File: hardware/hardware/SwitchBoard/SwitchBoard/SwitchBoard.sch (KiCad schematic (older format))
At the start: 36 parts, among them SW1 SW_SPDT, SW2 SW_SPDT, SW3 SW_SPDT, SW4 SW_SPDT, SW5 SW_SPDT, SW6 SW_SPDT, SW7 SW_SPDT, SW8 SW_SPDT, U1 BeagleBone_P8, U2 MCP23S08, U3 BeagleBone_P9, U4 NCP1117-3.3_SOT223

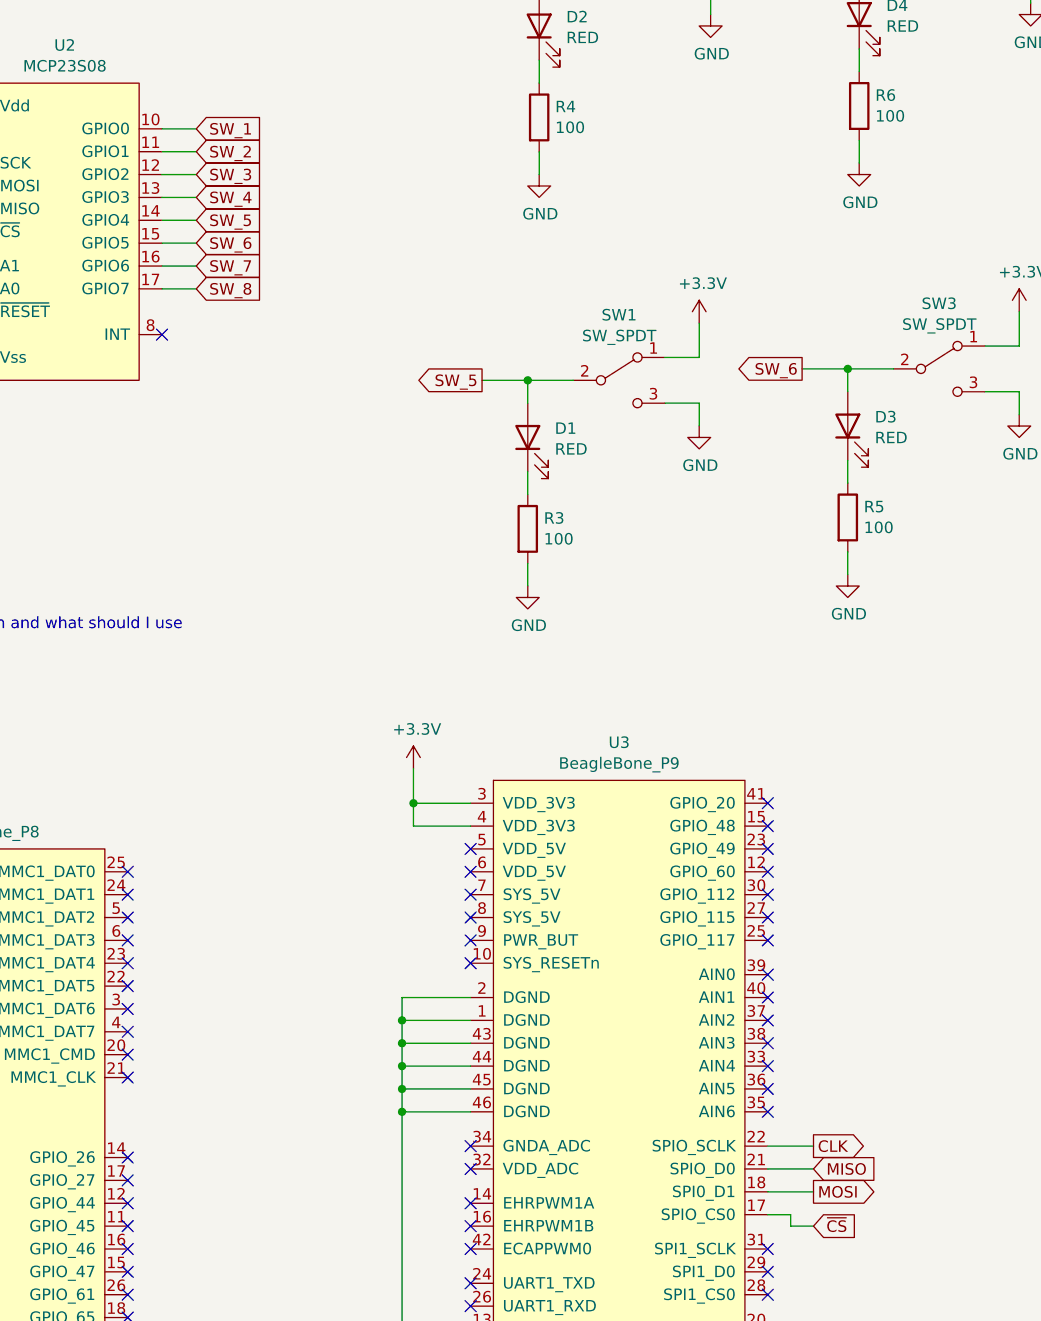
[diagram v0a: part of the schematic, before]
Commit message: More progress on switchboard
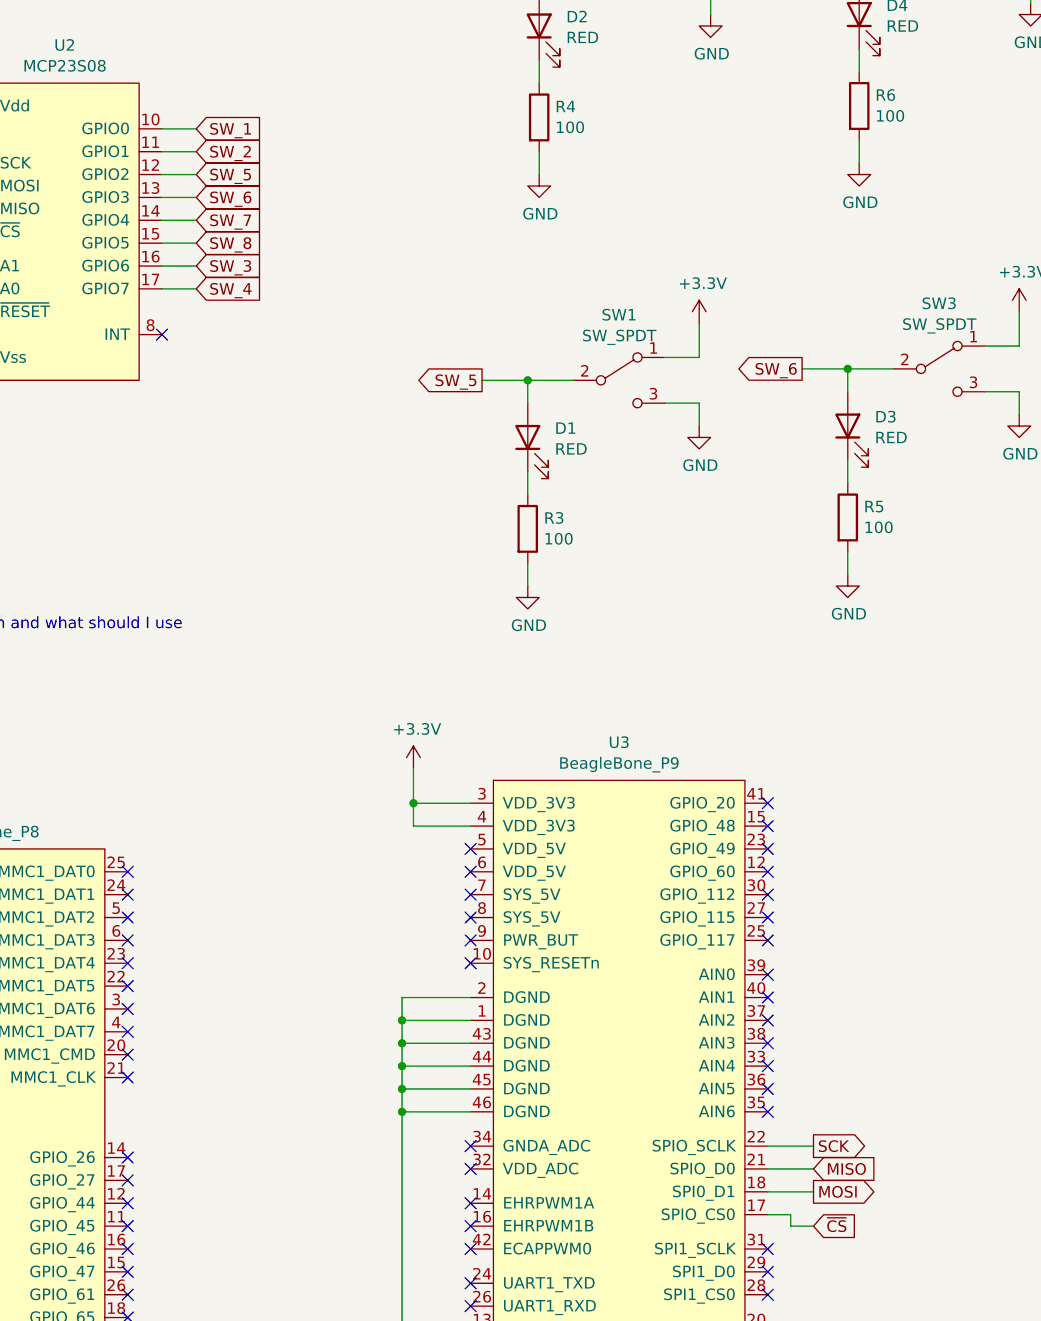
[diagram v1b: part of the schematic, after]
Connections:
- net CLK is gone; now on net SCK: U3.22 (SPIO_SCLK)
- net SW_3: now also U2.16 (GPIO6); no longer U2.12 (GPIO2)
- net SW_4: now also U2.17 (GPIO7); no longer U2.13 (GPIO3)
- net SW_5: now also U2.12 (GPIO2); no longer U2.14 (GPIO4)
- net SW_6: now also U2.13 (GPIO3); no longer U2.15 (GPIO5)
- net SW_7: now also U2.14 (GPIO4); no longer U2.16 (GPIO6)
- net SW_8: now also U2.15 (GPIO5); no longer U2.17 (GPIO7)
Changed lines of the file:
@@
 Text GLabel 3300 1900 2    50   Input ~ 0
 SW_2
+Text GLabel 3300 2400 2    50   Input ~ 0
+SW_3
+Text GLabel 3300 2500 2    50   Input ~ 0
+SW_4
 Text GLabel 3300 2000 2    50   Input ~ 0
-SW_3
+SW_5
 Text GLabel 3300 2100 2    50   Input ~ 0
-SW_4
+SW_6
 Text GLabel 3300 2200 2    50   Input ~ 0
-SW_5
+SW_7
 Text GLabel 3300 2300 2    50   Input ~ 0
-SW_6
-Text GLabel 3300 2400 2    50   Input ~ 0
-SW_7
-Text GLabel 3300 2500 2    50   Input ~ 0
 SW_8
 Wire Wire Line
@@
 Wire Wire Line
 	3300 1900 3150 1900
-Wire Wire Line
-	3150 2000 3300 2000
-Wire Wire Line
-	3150 2100 3300 2100
-Wire Wire Line
-	3150 2200 3300 2200
-Wire Wire Line
-	3150 2300 3300 2300
-Wire Wire Line
-	3150 2400 3300 2400
-Wire Wire Line
-	3150 2500 3300 2500
 $Comp
 L Switch:SW_SPDT SW2
@@
 $EndComp
 Text GLabel 6000 6250 2    50   Output ~ 0
-CLK
+SCK
 Text GLabel 6000 6350 2    50   Input ~ 0
 MISO
@@
 	1550 1600 1550 1550
 Connection ~ 1550 1600
+Wire Wire Line
+	3300 2500 3150 2500
+Wire Wire Line
+	3300 2400 3150 2400
+Wire Wire Line
+	3300 2300 3150 2300
+Wire Wire Line
+	3300 2200 3150 2200
+Wire Wire Line
+	3150 2100 3300 2100
+Wire Wire Line
+	3150 2000 3300 2000
 $EndSCHEMATC
